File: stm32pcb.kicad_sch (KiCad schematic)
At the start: 45 parts, among them J1 USB_C_Receptacle_USB2.0_16P, J2 Conn_01x04_Pin, J3 USB_C_Receptacle_USB2.0_16P, J4 Conn_01x12_Pin, J5 Conn_01x12_Pin, J6 Conn_01x12_Pin, J7 Conn_01x12_Pin, SW1 SW_Push_DPDT, SW2 SW_Push_DPDT, SW3 SW_Push_DPDT, SW4 SW_Push_DPDT, SW5 TS-1088-AR02016, U1 STM32F103C_8-B_Tx, U2 CH340C, U3 AMS1117-3.3, Y1 8MHz, Y2 32.768kHz

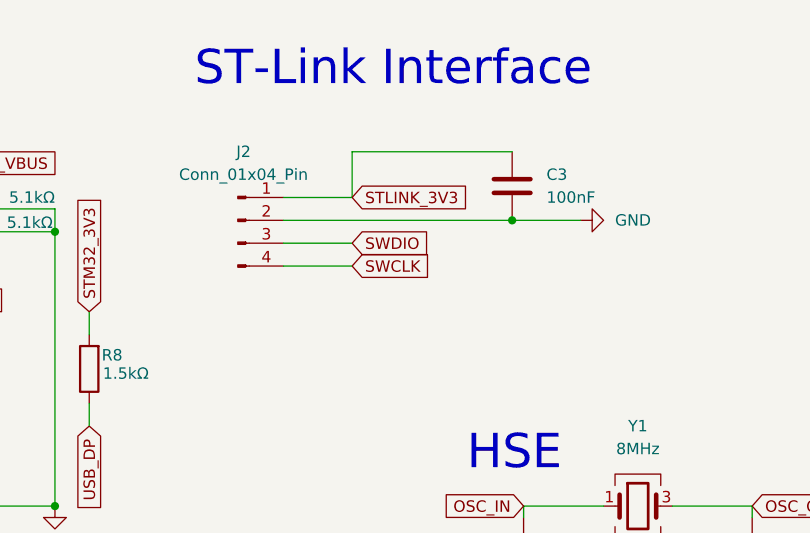
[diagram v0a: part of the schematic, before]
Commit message: update
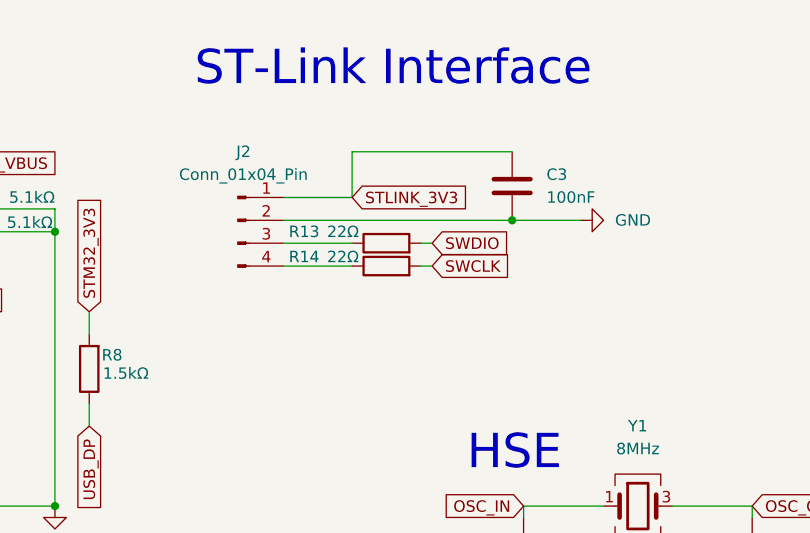
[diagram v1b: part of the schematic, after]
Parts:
- added R13, R14: 22Ω, Resistor_SMD:R_1206_3216Metric, symbol Device:R
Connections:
- net SWCLK: now also R14.2; no longer J2.4 (Pin_4)
- net SWDIO: now also R13.2; no longer J2.3 (Pin_3)
- new net: J2.3 (Pin_3), R13.1
- new net: J2.4 (Pin_4), R14.1
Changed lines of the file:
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@@
 	(wire
 		(pts
+			(xy 101.6 40.64) (xy 102.87 40.64)
+		)
+		(stroke
+			(width 0)
+			(type default)
+		)
+	)
+	(wire
+		(pts
 			(xy 116.84 257.81) (xy 123.19 257.81)
 		)
@@
 	(wire
 		(pts
+			(xy 101.6 38.1) (xy 102.87 38.1)
+		)
+		(stroke
+			(width 0)
+			(type default)
+		)
+	)
+	(wire
+		(pts
 			(xy 375.92 69.85) (xy 386.08 69.85)
 		)
@@
 		)
 	)
-	(global_label "SWCLK"
-		(shape input)
-		(at 93.98 40.64 0)
-		(fields_autoplaced yes)
-		(effects
-			(font
-				(size 1.27 1.27)
-			)
-			(justify left)
-		)
-		(property "Intersheetrefs" "${INTERSHEET_REFS}"
-			(at 103.1942 40.64 0)
-			(effects
-				(font
-					(size 1.27 1.27)
-				)
-				(justify left)
-				(hide yes)
-			)
-		)
-	)
 	(global_label "PB2_BOOT1"
 		(shape input)
@@
 		)
 	)
+	(global_label "SWCLK"
+		(shape input)
+		(at 102.87 40.64 0)
+		(fields_autoplaced yes)
+		(effects
+			(font
+				(size 1.27 1.27)
+			)
+			(justify left)
+		)
+		(property "Intersheetrefs" "${INTERSHEET_REFS}"
+			(at 112.0842 40.64 0)
+			(effects
+				(font
+					(size 1.27 1.27)
+				)
+				(justify left)
+				(hide yes)
+			)
+		)
+	)
 	(global_label "STM32_3V3"
 		(shape input)
@@
 		)
 	)
-	(global_label "SWDIO"
-		(shape input)
-		(at 93.98 38.1 0)
-		(fields_autoplaced yes)
-		(effects
-			(font
-				(size 1.27 1.27)
-			)
-			(justify left)
-		)
-		(property "Intersheetrefs" "${INTERSHEET_REFS}"
-			(at 102.8314 38.1 0)
-			(effects
-				(font
-					(size 1.27 1.27)
-				)
-				(justify left)
-				(hide yes)
-			)
-		)
-	)
 	(global_label "CH340_RX"
 		(shape input)
@@
 		)
 	)
+	(global_label "SWDIO"
+		(shape input)
+		(at 102.87 38.1 0)
+		(fields_autoplaced yes)
+		(effects
+			(font
+				(size 1.27 1.27)
+			)
+			(justify left)
+		)
+		(property "Intersheetrefs" "${INTERSHEET_REFS}"
+			(at 111.7214 38.1 0)
+			(effects
+				(font
+					(size 1.27 1.27)
+				)
+				(justify left)
+				(hide yes)
+			)
+		)
+	)
 	(global_label "CH340_RX"
 		(shape input)
@@
 	)
 	(symbol
+		(lib_id "Device:R")
+		(at 97.79 38.1 90)
+		(unit 1)
+		(exclude_from_sim no)
+		(in_bom yes)
+		(on_board yes)
+		(dnp no)
+		(property "Reference" "R13"
+			(at 88.646 36.83 90)
+			(effects
+				(font
+					(size 1.27 1.27)
+				)
+			)
+		)
+		(property "Value" "22Ω"
+			(at 92.964 36.83 90)
+			(effects
+				(font
+					(size 1.27 1.27)
+				)
+			)
+		)
+		(property "Footprint" "Resistor_SMD:R_1206_3216Metric"
+			(at 97.79 39.878 90)
+			(effects
+				(font
+					(size 1.27 1.27)
+				)
+				(hide yes)
+			)
+		)
+		(property "Datasheet" "~"
+			(at 97.79 38.1 0)
+			(effects
+				(font
+					(size 1.27 1.27)
+				)
+				(hide yes)
+			)
+		)
+		(property "Description" "Resistor"
+			(at 97.79 38.1 0)
+			(effects
+				(font
+					(size 1.27 1.27)
+				)
+				(hide yes)
+			)
+		)
+		(pin "1"
+		)
+		(pin "2"
+		)
+		(instances
+			(project "stm32pcb"
+				(path "/deb2f888-ee5e-42ae-a295-95cf39931a97"
+					(reference "R13")
+					(unit 1)
+				)
+			)
+		)
+	)
+	(symbol
 		(lib_id "Device:C")
 		(at 69.85 240.03 0)
@@
 					(unit 1)
 				)
+			)
+		)
+	)
+	(symbol
+		(lib_id "Device:R")
+		(at 97.79 40.64 90)
+		(unit 1)
+		(exclude_from_sim no)
+		(in_bom yes)
+		(on_board yes)
+		(dnp no)
+		(property "Reference" "R14"
+			(at 88.646 39.624 90)
+			(effects
+				(font
+					(size 1.27 1.27)
+				)
+			)
+		)
+		(property "Value" "22Ω"
+			(at 92.964 39.624 90)
+			(effects
+				(font
+					(size 1.27 1.27)
+				)
+			)
+		)
+		(property "Footprint" "Resistor_SMD:R_1206_3216Metric"
+			(at 97.79 42.418 90)
+			(effects
+				(font
+					(size 1.27 1.27)
+				)
+				(hide yes)
+			)
+		)
+		(property "Datasheet" "~"
+			(at 97.79 40.64 0)
+			(effects
+				(font
+					(size 1.27 1.27)
+				)
+				(hide yes)
+			)
+		)
+		(property "Description" "Resistor"
+			(at 97.79 40.64 0)
+			(effects
+				(font
+					(size 1.27 1.27)
+				)
+				(hide yes)
+			)
+		)
+		(pin "1"
+		)
+		(pin "2"
+		)
+		(instances
+			(project "stm32pcb"
+				(path "/deb2f888-ee5e-42ae-a295-95cf39931a97"
+					(reference "R14")
+					(unit 1)
+				)
